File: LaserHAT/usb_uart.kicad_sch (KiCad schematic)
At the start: 9 parts

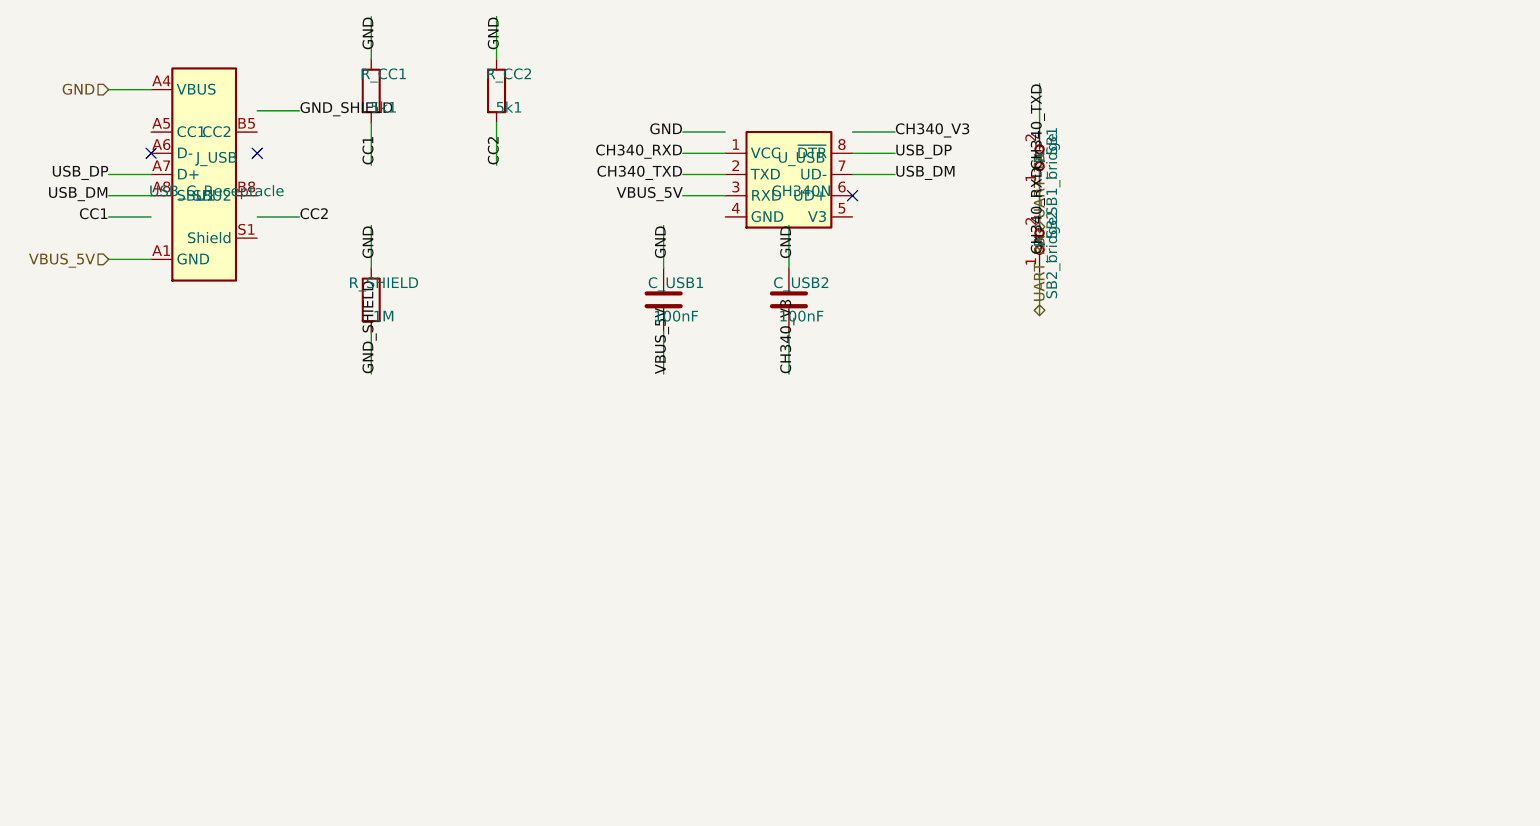
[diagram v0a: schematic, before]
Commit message: Updates with lots of manual work
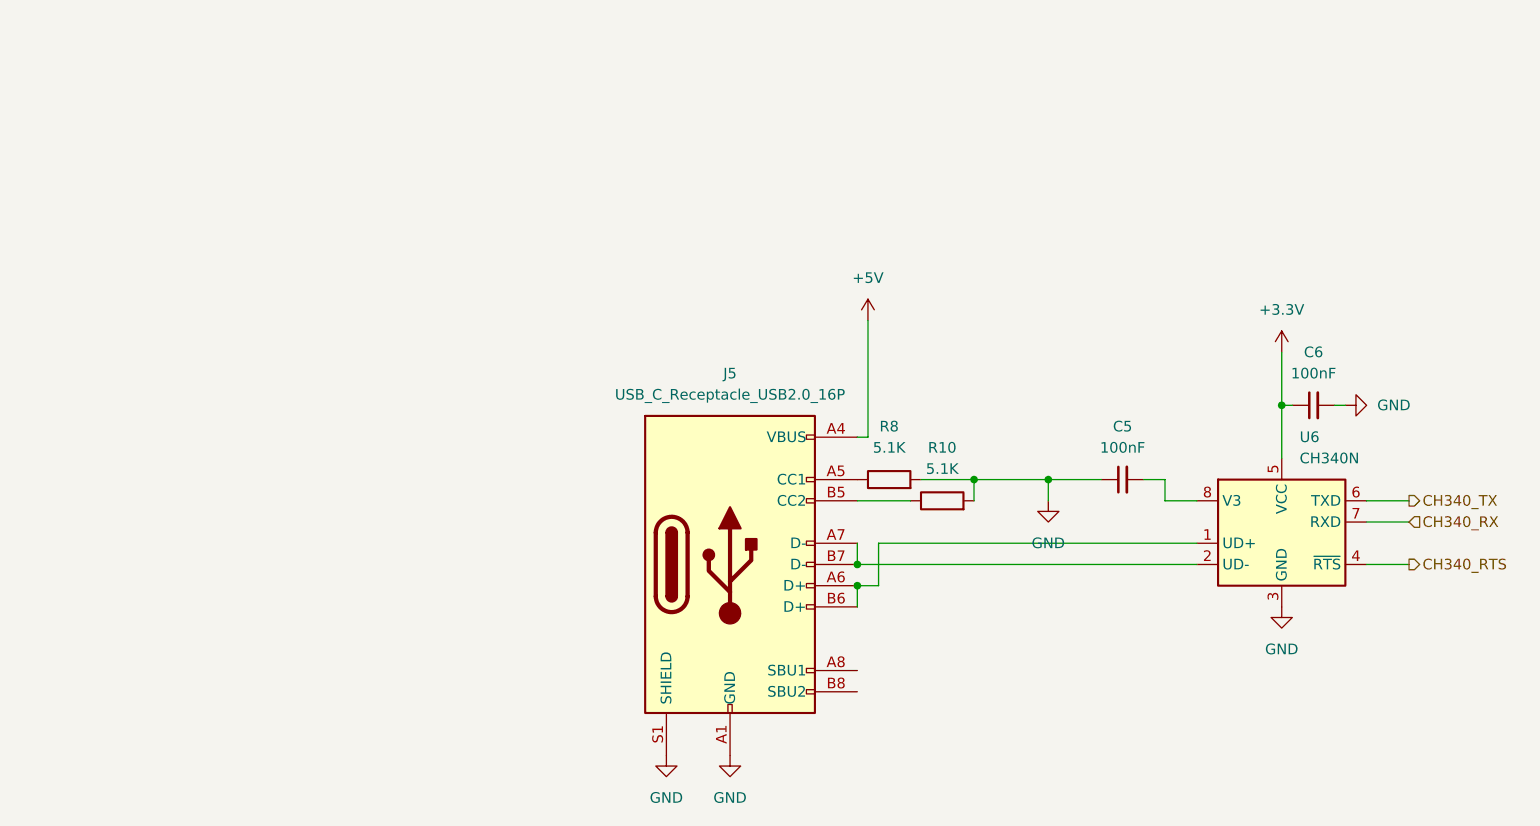
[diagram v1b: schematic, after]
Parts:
- removed C_USB1, C_USB2: 100nF, Capacitor_SMD:C_0402_1005Metric, symbol Device:C
- removed J_USB: USB_C_Receptacle, Connector_USB:USB_C_Receptacle_GCT_USB4125, symbol Connector_USB:USB_C_Receptacle_USB2.0
- removed R_CC1, R_CC2: 5k1, Resistor_SMD:R_0402_1005Metric, symbol Device:R
- removed R_SHIELD: 1M, Resistor_SMD:R_0402_1005Metric, symbol Device:R
- removed SB1: SB1_bridge, Jumper:SolderJumper-2_P1.3mm_Open_RoundedPad1.0x1.5mm, symbol Jumper:SolderJumper_2_Open
- removed SB2: SB2_bridge, Jumper:SolderJumper-2_P1.3mm_Open_RoundedPad1.0x1.5mm, symbol Jumper:SolderJumper_2_Open
- removed U_USB: CH340N, Package_SO:SOIC-8_3.9x4.9mm_P1.27mm, symbol Interface_USB:CH340N
- added C5, C6: 100nF, Capacitor_SMD:C_0402_1005Metric, symbol Device:C_Small
- added J5: USB_C_Receptacle_USB2.0_16P, symbol Connector:USB_C_Receptacle_USB2.0_16P
- added R10, R8: 5.1K, Resistor_SMD:R_0402_1005Metric, symbol Device:R
- added U6: CH340N, Package_SO:JEITA_SOIC-8_3.9x4.9mm_P1.27mm, symbol Interface_USB:CH340N
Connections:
- net GND: now also C5.1, C6.2, J5.A1 (GND), J5.A12 (GND), J5.B1 (GND), J5.B12 (GND), J5.S1 (SHIELD), R10.2, R8.2, U6.3 (GND)
- new net: J5.B5 (CC2), R10.1
- new net: J5.A6 (D+), J5.B6 (D+), U6.1 (UD+)
- new net: J5.A7 (D-), J5.B7 (D-), U6.2 (UD-)
- new net: C5.2, U6.8 (V3)
- new net: J5.A5 (CC1), R8.1
- new net +3.3V: C6.1, U6.5 (VCC)
- new net +5V: J5.A4 (VBUS), J5.A9 (VBUS), J5.B4 (VBUS), J5.B9 (VBUS)
- new net CH340_RTS: U6.4 (~{RTS})
- new net CH340_RX: U6.7 (RXD)
- new net CH340_TX: U6.6 (TXD)
- no-connect marks 3 -> 0
